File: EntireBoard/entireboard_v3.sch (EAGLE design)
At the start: 50 parts, among them J1 MF-CON-2.54mm-01x09, P1 0532610271, U1 TPS7A0508PDBVRDBV0005A_M, U2 RHD2216_QFN

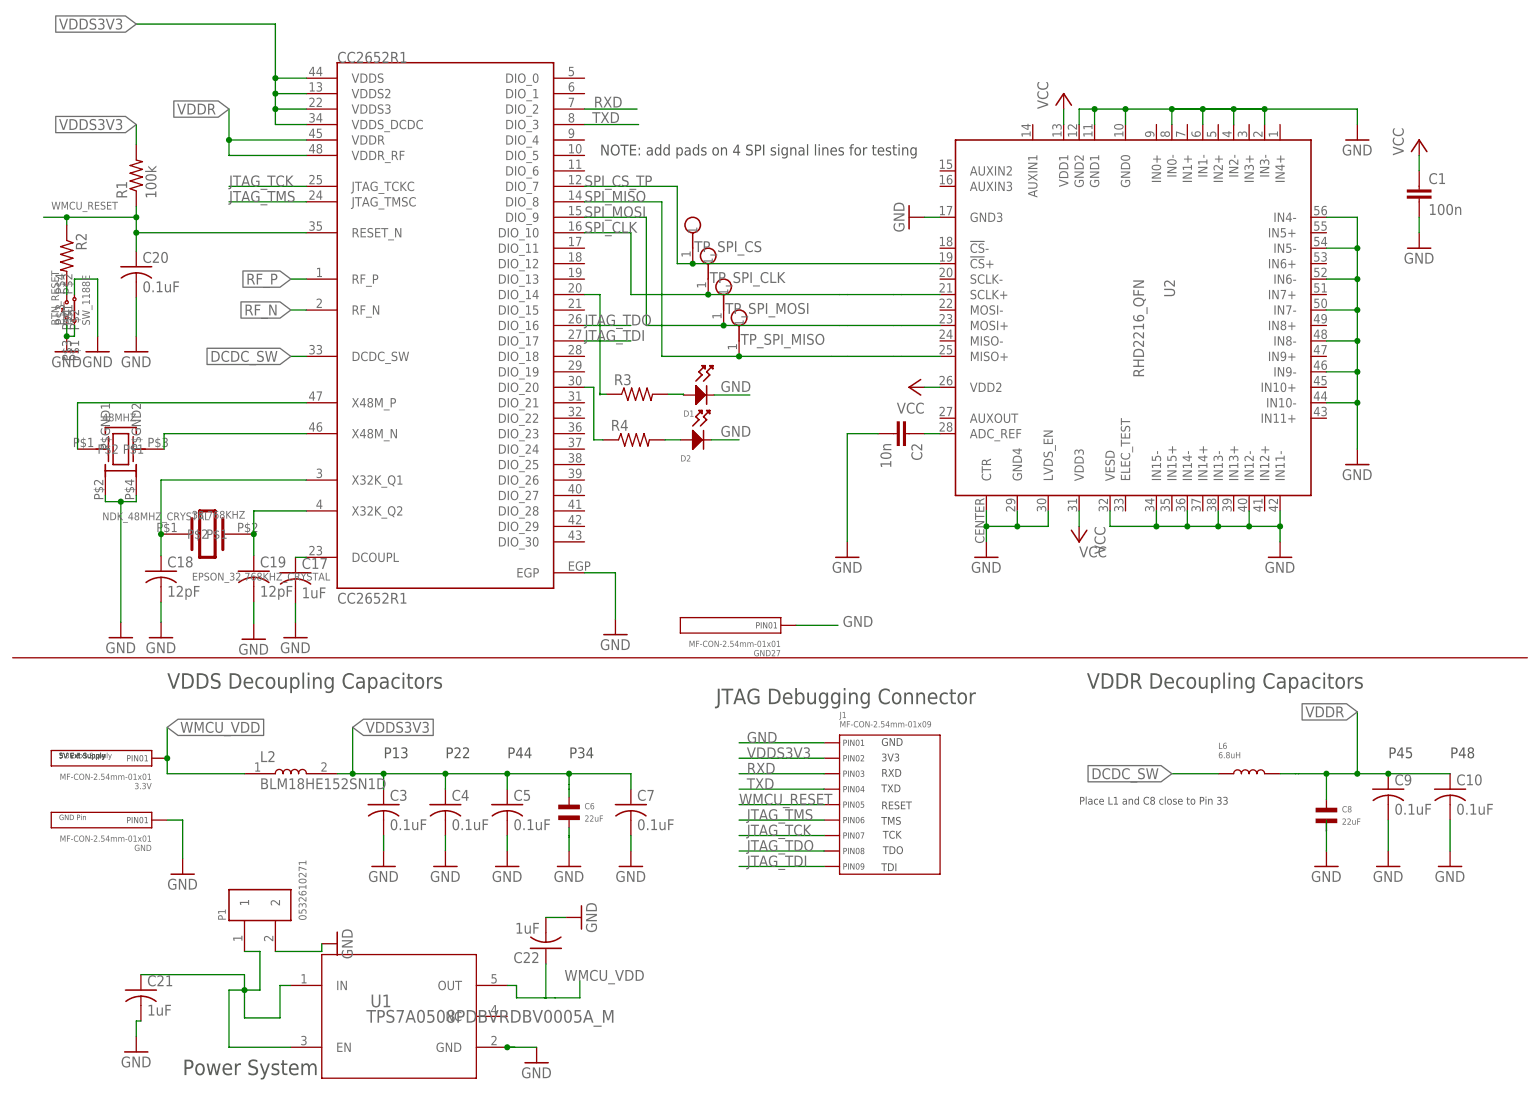
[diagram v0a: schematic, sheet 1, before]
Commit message: version 3!! 4x4cm
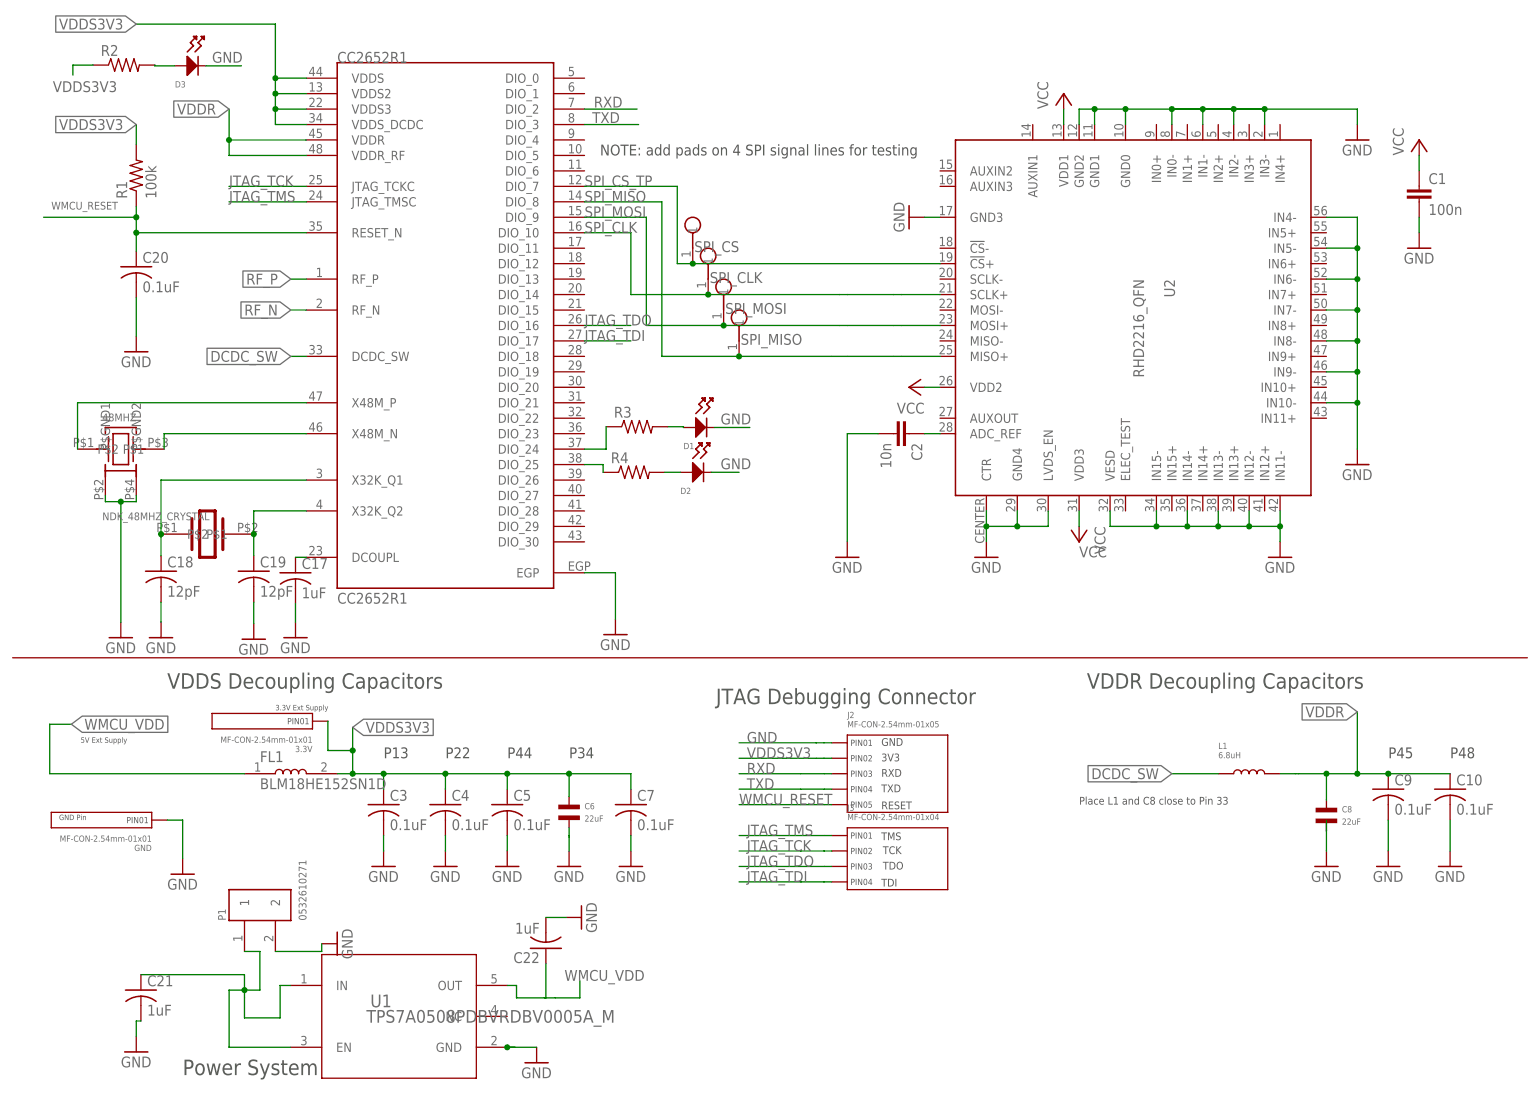
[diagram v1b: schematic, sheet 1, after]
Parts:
- removed BTN_RESET: SW_1188E, AxonMobile:SW_1188E
- removed GND27: MF-CON-2.54mm-01x01, AxonMobile:CON_01X01_PTH_2.54MM
- removed J1: MF-CON-2.54mm-01x09, MF_Connectors:CON_01X09_PTH_2.54MM
- removed L6: 6.8uH, MF_Passives:INDUCTOR_0603
- added D3: (no value), MF_LEDs:LED_SINGLE-0603
- added FL1: BLM18HE152SN1D, BLM18HE152SN1D:BLM18HE152SN1D
- added J2: MF-CON-2.54mm-01x05, MF_Connectors:CON_01X05_PTH_2.54MM
- added J3: MF-CON-2.54mm-01x04, MF_Connectors:CON_01X04_PTH_2.54MM
- C11, C12, C13, C14, C15, C16: device adafruit:C-USC0402 -> MF_Passives:CAPACITOR_NP_0402
- L1: value 2.4nH -> 6.8uH; device rcl-2:L-USL0201 -> MF_Passives:INDUCTOR_0603
- L2: value BLM18HE152SN1D -> 2nH; device BLM18HE152SN1D:BLM18HE152SN1D -> MF_Passives:INDUCTOR_0402
- L3, L4: device rcl-2:L-USL0201 -> MF_Passives:INDUCTOR_0402
- L5: value 2nH -> 2.4nH; device rcl-2:L-USL0201 -> MF_Passives:INDUCTOR_0402
- renumbered TP_SPI_CLK to SPI_CLK, TP_SPI_CS to SPI_CS, TP_SPI_MISO to SPI_MISO, TP_SPI_MOSI to SPI_MOSI
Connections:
- removed net N$25: CC2652R1.DIO_20, R4.1
- new net N$17: CC2652R1.DIO_24, R3.1
- net DCDC_SW: now also L1.P$1; no longer L6.P$1
- net GND: now also C13.P$2, C15.P$2, C16.P$2, D3.CATHODE, J2.PIN1; no longer BTN_RESET.P$1, BTN_RESET.P$2, BTN_RESET.P$3, C13.2, C15.2, C16.2, GND27.PIN1, J1.PIN1
- net JTAG_TCK: now also J3.PIN2; no longer J1.PIN7
- net JTAG_TDI: now also J3.PIN4; no longer J1.PIN9
- net JTAG_TDO: now also J3.PIN3; no longer J1.PIN8
- net JTAG_TMS: now also J3.PIN1; no longer J1.PIN6
- net N$11: now also C11.P$2; no longer C11.2
- net N$12: now also C16.P$1, L5.P$2; no longer C16.1, L1.2
- net N$13: now also CC2652R1.DIO_25, R4.1; no longer CC2652R1.DIO_14, R3.1
- net N$16: now also D3.ANODE; no longer BTN_RESET.P$4
- net N$6: now also C11.P$1, C12.P$2; no longer C11.1, C12.2
- net N$7: now also C12.P$1, L2.P$2; no longer C12.1, L5.2
- net N$8: now also C13.P$1, L2.P$1, L3.P$2; no longer C13.1, L3.2, L5.1
- net N$9: now also C14.P$2, L3.P$1, L4.P$2; no longer C14.2, L3.1, L4.2
- net RF_N: now also C15.P$1, L4.P$1; no longer C15.1, L4.1
- net RF_P: now also C14.P$1, L5.P$1; no longer C14.1, L1.1
- net RXD: now also J2.PIN3; no longer J1.PIN3
- net TXD: now also J2.PIN4; no longer J1.PIN4
- net VDDR: now also L1.P$2; no longer L6.P$2
- net VDDS3V3: now also 3.3V.PIN1, FL1.2, J2.PIN2, R2.1; no longer J1.PIN2, L2.2
- net WMCU_RESET: now also J2.PIN5; no longer J1.PIN5, R2.1
- net WMCU_VDD: now also FL1.1; no longer 3.3V.PIN1, L2.1
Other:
- moved on the sheet: 3.3V, D1, D2, R2, R3, R4

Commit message: final (??) board v3
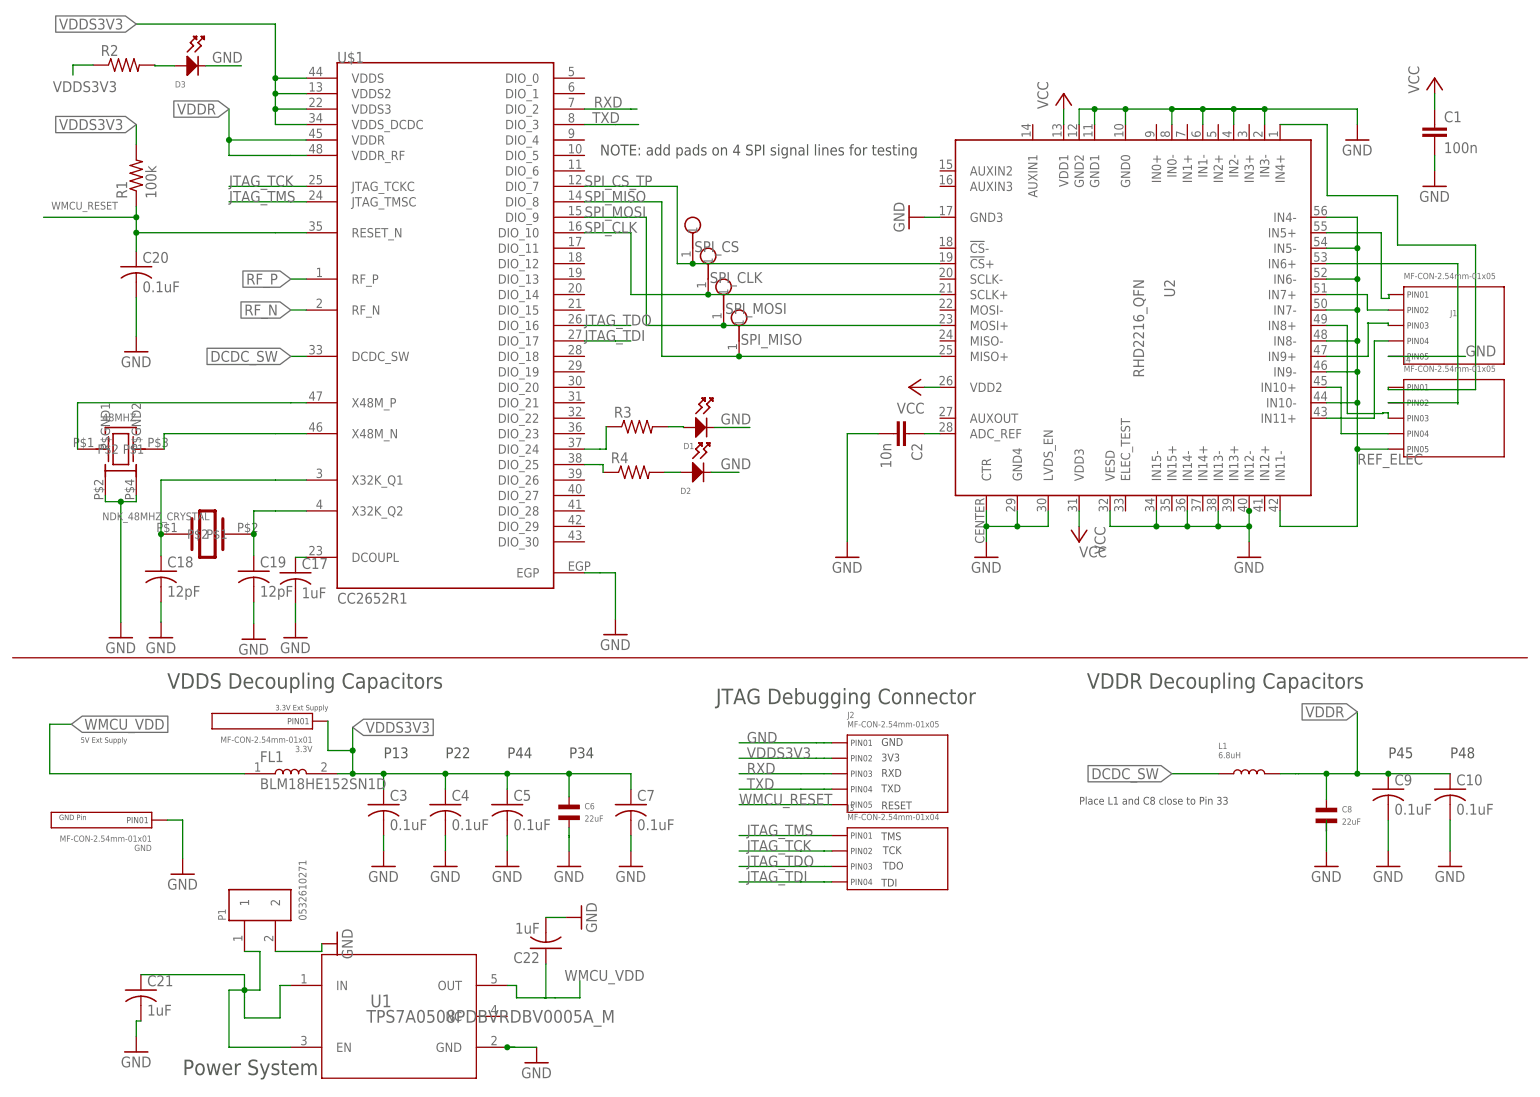
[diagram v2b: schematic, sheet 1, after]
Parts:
- added J1, J4: MF-CON-2.54mm-01x05, MF_Connectors:CON_01X05_PTH_2.54MM
- renumbered CC2652R1 to U$1
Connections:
- new net N$18: J1.PIN4, U2.IN11+
- new net N$19: J4.PIN4, U2.IN10+
- new net N$20: J1.PIN3, U2.IN9+
- new net N$21: J4.PIN3, U2.IN8+
- new net N$22: J1.PIN2, U2.IN7+
- new net N$23: J4.PIN2, U2.IN6+
- new net N$24: J1.PIN1, U2.IN5+
- new net N$25: J4.PIN1, U2.IN4+
- new net REF_ELEC: J4.PIN5, U2.IN10-, U2.IN11-, U2.IN4-, U2.IN5-, U2.IN6-, U2.IN7-, U2.IN8-, U2.IN9-
- net GND: now also J1.PIN5; no longer U2.IN10-, U2.IN11-, U2.IN4-, U2.IN5-, U2.IN6-, U2.IN7-, U2.IN8-, U2.IN9-
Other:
- moved on the sheet: C1
